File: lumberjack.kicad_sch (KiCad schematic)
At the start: 159 parts, among them J1 USB, J2 AVR_ISP_6, J3 JST, J4 JST, SW1 RESET, SW2 BOOT, U1 ATMEGA328-PU, Y1 16MHz

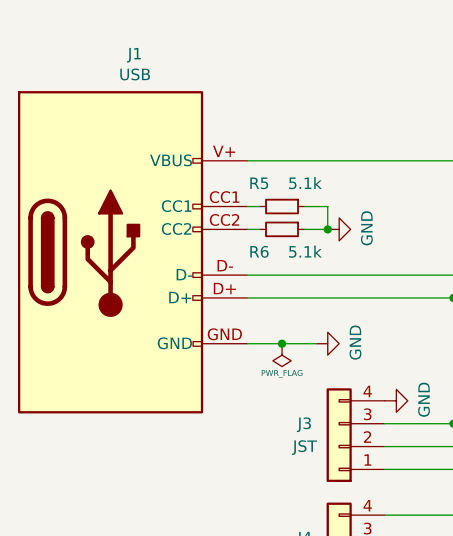
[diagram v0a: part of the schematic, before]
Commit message: 130423 Update
Finished about 75% of the routing.
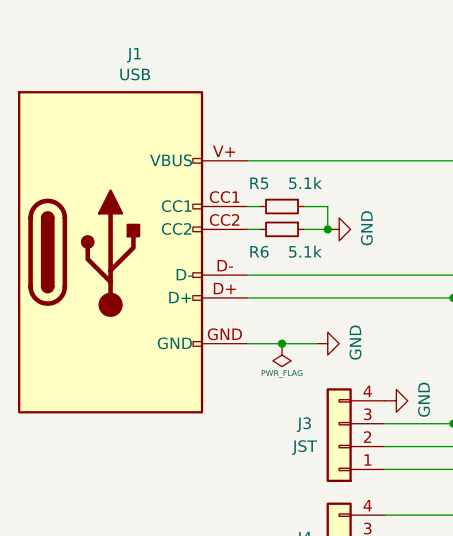
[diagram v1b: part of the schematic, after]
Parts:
- MX1, MX10, MX11, MX12, MX13, MX14, MX15, MX16, MX17, MX18, MX19, MX2, MX20, MX21, MX22, MX23, MX24, MX25, MX26, MX27, MX28, MX29, MX3, MX30, MX31, MX32, MX33, MX34, MX35, MX36, MX37, MX38, MX39, MX4, MX40, MX41, MX42, MX43, MX44, MX45, MX46, MX47, MX48, MX49, MX5, MX50, MX51, MX52, MX53, MX54, MX55, MX56, MX57, MX58, MX59, MX6, MX60, MX7, MX9: footprint lumberjack:MX_Alps_Choc -> Library:Lumberjack CherryMX_Choc_v1v2_Hotswap Single Side
- MX8: footprint lumberjack:MX_Alps_Choc_NTHSTH -> Library:Lumberjack CherryMX_Choc_v1v2_Hotswap Single Side
